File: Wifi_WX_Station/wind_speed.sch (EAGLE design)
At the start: 8 parts, among them T1 MMBT3904

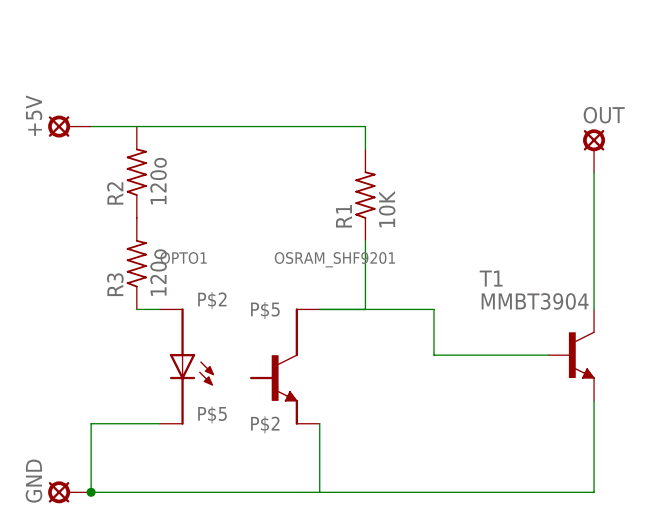
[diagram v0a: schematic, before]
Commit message: updated BOM with all prices- As Checked in to BATCH PCB
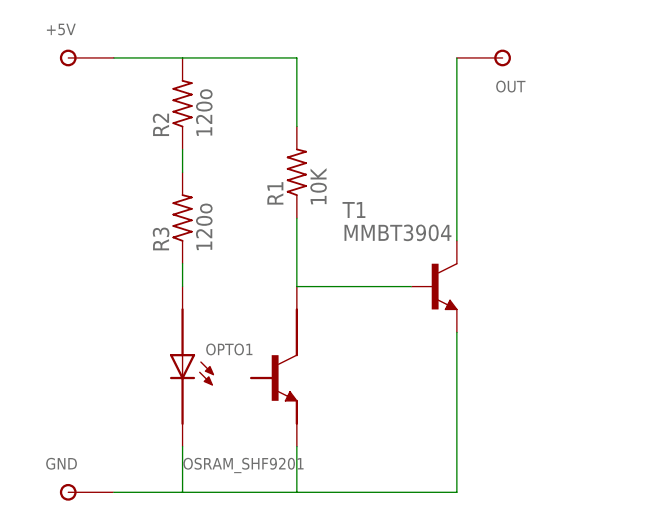
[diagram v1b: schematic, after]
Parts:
- +5V, GND, OUT: value LSP10 -> TPSOL; device solpad:LSP10 -> wifi_WX:TPSOL
- OPTO1: device 1AA_Stofer:OSRAM_SHF9201 -> wifi_WX:OSRAM_SHF9201
- R1: device rcl:R-US_R0805 -> rcl:R-US_R0603
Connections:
- net N$2: now also GND.P$1; no longer GND.MP
- net N$3: now also +5V.P$1; no longer +5V.MP
- net N$4: now also OUT.P$1; no longer OUT.MP
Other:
- moved on the sheet: R1, R2, R3, T1
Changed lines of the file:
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@@
 </classes>
 <parts>
-<part name="OPTO1" library="1AA_Stofer" deviceset="OSRAM_SHF9201" device=""/>
+<part name="OPTO1" library="wifi_WX" deviceset="OSRAM_SHF9201" device=""/>
 <part name="T1" library="transistor" deviceset="BC846" device="" value="MMBT3904"/>
-<part name="R1" library="rcl" deviceset="R-US_" device="R0805" value="10K"/>
-<part name="+5V" library="solpad" deviceset="LSP10" device=""/>
-<part name="GND" library="solpad" deviceset="LSP10" device=""/>
-<part name="OUT" library="solpad" deviceset="LSP10" device=""/>
+<part name="R1" library="rcl" deviceset="R-US_" device="R0603" value="10K"/>
 <part name="R2" library="rcl" deviceset="R-US_" device="R0603" value="120o"/>
 <part name="R3" library="rcl" deviceset="R-US_" device="R0603" value="120o"/>
+<part name="+5V" library="wifi_WX" deviceset="TP" device="SOL"/>
+<part name="GND" library="wifi_WX" deviceset="TP" device="SOL"/>
+<part name="OUT" library="wifi_WX" deviceset="TP" device="SOL"/>
 </parts>
 <sheets>
@@
 </plain>
 <instances>
-<instance part="OPTO1" gate="G$1" x="101.6" y="60.96"/>
-<instance part="T1" gate="G$1" x="139.7" y="63.5"/>
-<instance part="R1" gate="G$1" x="116.84" y="81.28" rot="R90"/>
-<instance part="+5V" gate="1" x="83.82" y="88.9" rot="R90"/>
-<instance part="GND" gate="1" x="83.82" y="48.26" rot="R90"/>
-<instance part="OUT" gate="1" x="142.24" y="86.36"/>
-<instance part="R2" gate="G$1" x="91.44" y="83.82" rot="R90"/>
-<instance part="R3" gate="G$1" x="91.44" y="73.66" rot="R90"/>
+<instance part="OPTO1" gate="G$1" x="101.6" y="60.96" smashed="yes">
+<attribute name="NAME" x="99.06" y="63.5" size="1.27" layer="95"/>
+<attribute name="VALUE" x="96.52" y="50.8" size="1.27" layer="96"/>
+</instance>
+<instance part="T1" gate="G$1" x="124.46" y="71.12"/>
+<instance part="R1" gate="G$1" x="109.22" y="83.82" rot="R90"/>
+<instance part="R2" gate="G$1" x="96.52" y="91.44" rot="R90"/>
+<instance part="R3" gate="G$1" x="96.52" y="78.74" rot="R90"/>
+<instance part="+5V" gate="G$1" x="83.82" y="96.52"/>
+<instance part="GND" gate="G$1" x="83.82" y="48.26"/>
+<instance part="OUT" gate="G$1" x="132.08" y="96.52" rot="R180"/>
 </instances>
 <busses>
@@
 <pinref part="R1" gate="G$1" pin="1"/>
 <pinref part="OPTO1" gate="G$1" pin="C"/>
-<wire x1="116.84" y1="76.2" x2="116.84" y2="68.58" width="0.1524" layer="91"/>
-<wire x1="116.84" y1="68.58" x2="111.76" y2="68.58" width="0.1524" layer="91"/>
-<wire x1="111.76" y1="68.58" x2="124.46" y2="68.58" width="0.1524" layer="91"/>
-<wire x1="124.46" y1="68.58" x2="124.46" y2="63.5" width="0.1524" layer="91"/>
+<wire x1="109.22" y1="78.74" x2="109.22" y2="71.12" width="0.1524" layer="91"/>
+<wire x1="109.22" y1="71.12" x2="121.92" y2="71.12" width="0.1524" layer="91"/>
 <pinref part="T1" gate="G$1" pin="B"/>
-<wire x1="124.46" y1="63.5" x2="137.16" y2="63.5" width="0.1524" layer="91"/>
 </segment>
 </net>
@@
 <segment>
 <pinref part="OPTO1" gate="G$1" pin="E"/>
-<wire x1="111.76" y1="55.88" x2="111.76" y2="48.26" width="0.1524" layer="91"/>
+<wire x1="109.22" y1="53.34" x2="109.22" y2="48.26" width="0.1524" layer="91"/>
 <pinref part="T1" gate="G$1" pin="E"/>
-<wire x1="111.76" y1="48.26" x2="142.24" y2="48.26" width="0.1524" layer="91"/>
-<wire x1="142.24" y1="48.26" x2="142.24" y2="58.42" width="0.1524" layer="91"/>
+<wire x1="109.22" y1="48.26" x2="127" y2="48.26" width="0.1524" layer="91"/>
+<wire x1="127" y1="48.26" x2="127" y2="66.04" width="0.1524" layer="91"/>
 <pinref part="OPTO1" gate="G$1" pin="CATH"/>
-<wire x1="111.76" y1="48.26" x2="86.36" y2="48.26" width="0.1524" layer="91"/>
-<wire x1="86.36" y1="48.26" x2="86.36" y2="55.88" width="0.1524" layer="91"/>
-<wire x1="86.36" y1="55.88" x2="93.98" y2="55.88" width="0.1524" layer="91"/>
-<pinref part="GND" gate="1" pin="MP"/>
-<junction x="86.36" y="48.26"/>
+<wire x1="109.22" y1="48.26" x2="96.52" y2="48.26" width="0.1524" layer="91"/>
+<wire x1="88.9" y1="48.26" x2="96.52" y2="48.26" width="0.1524" layer="91"/>
+<wire x1="96.52" y1="48.26" x2="96.52" y2="53.34" width="0.1524" layer="91"/>
+<pinref part="GND" gate="G$1" pin="P$1"/>
 </segment>
 </net>
 <net name="N$3" class="0">
 <segment>
-<wire x1="86.36" y1="88.9" x2="91.44" y2="88.9" width="0.1524" layer="91"/>
+<wire x1="88.9" y1="96.52" x2="96.52" y2="96.52" width="0.1524" layer="91"/>
 <pinref part="R1" gate="G$1" pin="2"/>
-<wire x1="91.44" y1="88.9" x2="116.84" y2="88.9" width="0.1524" layer="91"/>
-<wire x1="116.84" y1="88.9" x2="116.84" y2="86.36" width="0.1524" layer="91"/>
-<pinref part="+5V" gate="1" pin="MP"/>
+<wire x1="96.52" y1="96.52" x2="109.22" y2="96.52" width="0.1524" layer="91"/>
+<wire x1="109.22" y1="96.52" x2="109.22" y2="88.9" width="0.1524" layer="91"/>
 <pinref part="R2" gate="G$1" pin="2"/>
+<pinref part="+5V" gate="G$1" pin="P$1"/>
 </segment>
 </net>
@@
 <segment>
 <pinref part="T1" gate="G$1" pin="C"/>
-<wire x1="142.24" y1="68.58" x2="142.24" y2="83.82" width="0.1524" layer="91"/>
-<pinref part="OUT" gate="1" pin="MP"/>
+<wire x1="127" y1="76.2" x2="127" y2="96.52" width="0.1524" layer="91"/>
+<pinref part="OUT" gate="G$1" pin="P$1"/>
 </segment>
 </net>
@@
 <segment>
 <pinref part="OPTO1" gate="G$1" pin="AN"/>
-<wire x1="91.44" y1="68.58" x2="93.98" y2="68.58" width="0.1524" layer="91"/>
+<wire x1="96.52" y1="73.66" x2="96.52" y2="71.12" width="0.1524" layer="91"/>
 <pinref part="R3" gate="G$1" pin="1"/>
 </segment>
@@
 <pinref part="R2" gate="G$1" pin="1"/>
 <pinref part="R3" gate="G$1" pin="2"/>
+<wire x1="96.52" y1="86.36" x2="96.52" y2="83.82" width="0.1524" layer="91"/>
 </segment>
 </net>
